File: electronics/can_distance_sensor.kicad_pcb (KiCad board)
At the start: 4 copper layers, 39.4 x 47.6 mm, 78 parts, among them J1 USB_B_Micro, J2 Conn_ARM_JTAG_SWD_10, J4 Conn_01x02_Socket, J5 Conn_01x04, Q1 IRLML6401, SW1 PTS645SK50SMTR92LFS, U1 USBLC6-2SC6, U2 STM32F446RETx, U3 LM1117DT-ADJ, U4 AOZ1280CI, U5 VL53L3CXV0DH/1, U6 TCAN1043xDxQ1, Y1 Crystal_GND24

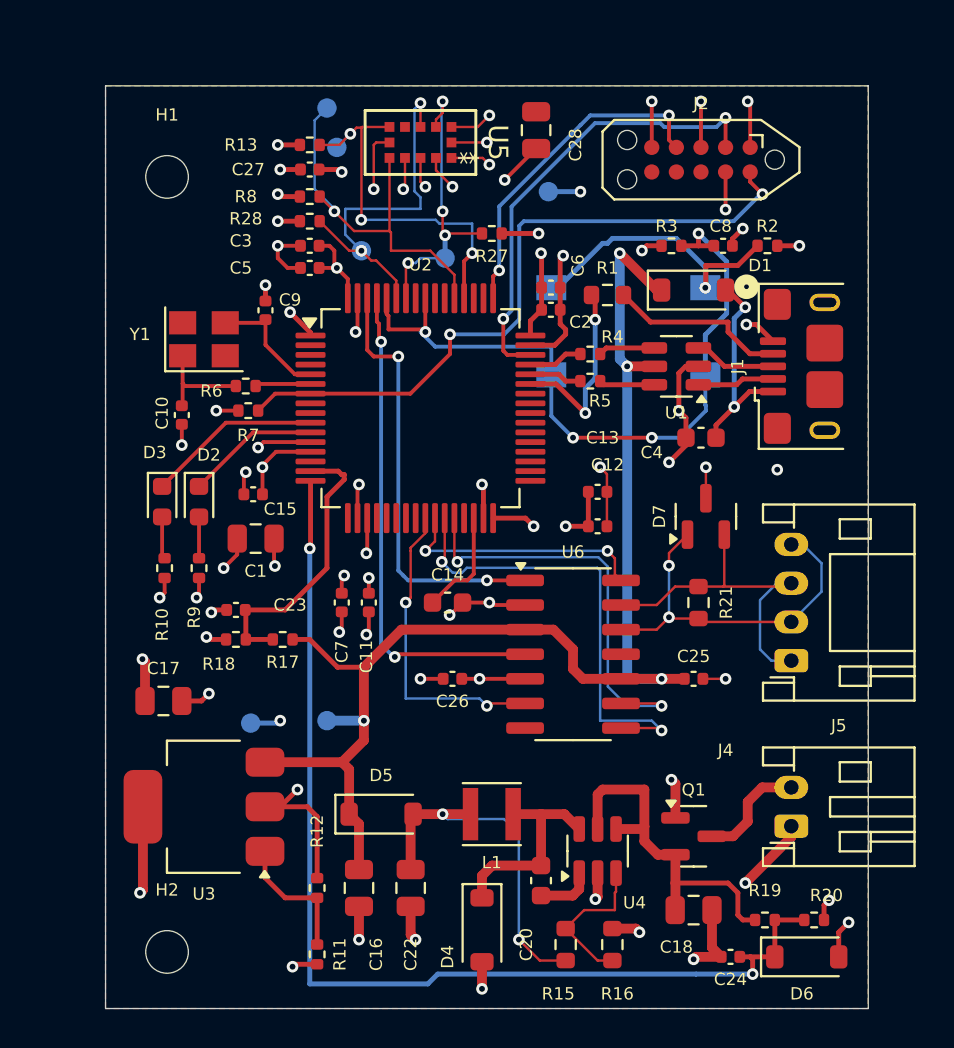
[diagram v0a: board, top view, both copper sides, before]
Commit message: Ordered this version.
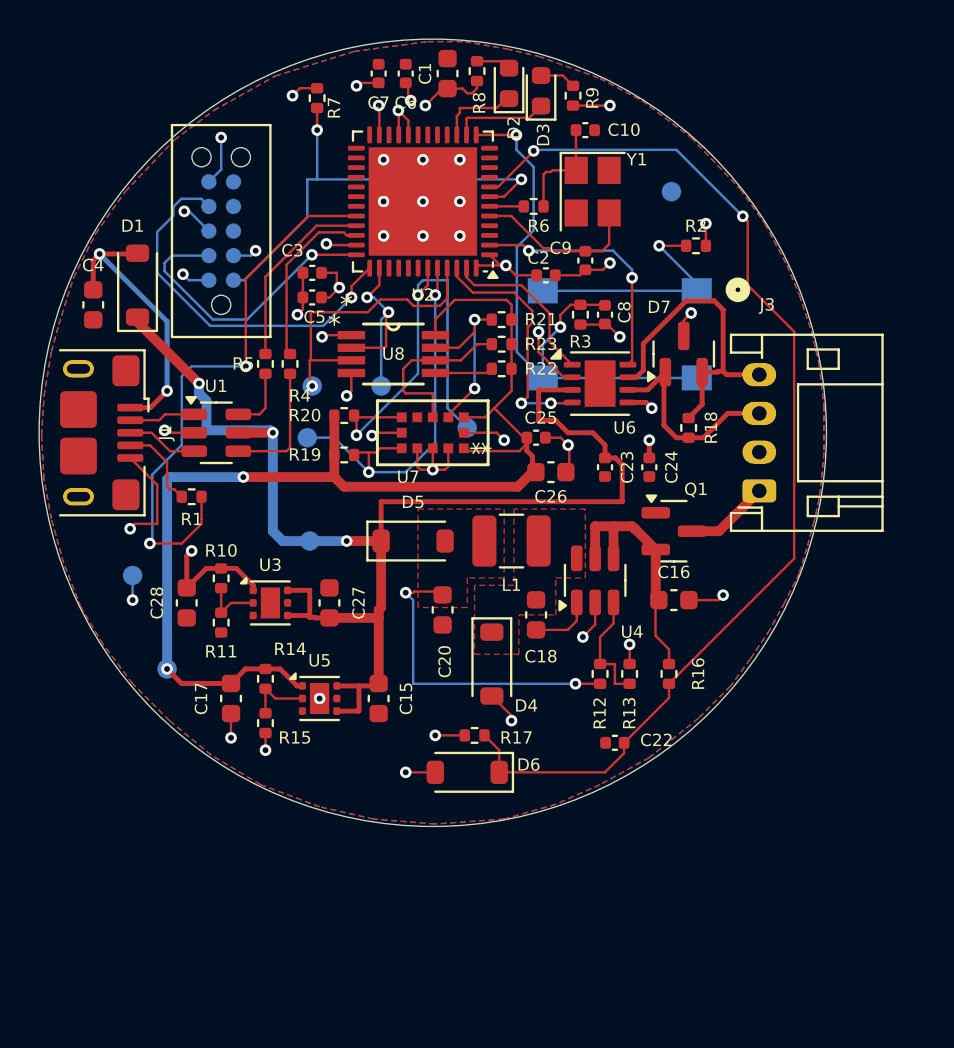
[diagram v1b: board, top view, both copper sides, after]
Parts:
- removed C11, C12, C13: 0.1u, Capacitor_SMD:C_0402_1005Metric
- removed C14: 2.2u, Capacitor_SMD:C_0603_1608Metric
- removed the C16 at (190.2, 129.2)
- removed the C23 at (183.9, 114.8)
- removed H1, H2: MountingHole, MountingHole:MountingHole_2.2mm_M2
- removed J4: Conn_01x02_Socket, Connector_JST:JST_PH_S2B-PH-K_1x02_P2.00mm_Horizontal
- removed the R12 at (188.1, 129.2)
- removed the R17 at (186.3, 116.3)
- removed the R18 at (183.9, 116.3)
- added C27: 4.7u, Capacitor_SMD:C_0603_1608Metric, F.Cu at (188.7, 114.4)
- added C28: 4.7u, Capacitor_SMD:C_0603_1608Metric, F.Cu at (181.4, 114.4)
- added R10: 5k, Resistor_SMD:R_0402_1005Metric, F.Cu at (183.1, 113.2)
- added R14: 4.09k, Resistor_SMD:R_0402_1005Metric, F.Cu at (185.4, 118.4)
- added R15: 1k, Resistor_SMD:R_0402_1005Metric, F.Cu at (185.4, 120.7)
- added R22: 10K, Resistor_SMD:R_0402_1005Metric, F.Cu at (197.6, 102.4)
- added TP8: TestPoint, TestPoint:TestPoint_Pad_D1.0mm, B.Cu at (180.3, 117.9)
- added U5: TLV75801PDRV, Package_SON:WSON-6-1EP_2x2mm_P0.65mm_EP1x1.6mm, F.Cu at (188.2, 119.4)
- added U8: TCA9509DGKR, footprints:DGK8, F.Cu at (192.0, 101.6)
- C1: footprint Capacitor_SMD:C_0805_2012Metric -> Capacitor_SMD:C_0603_1608Metric
- C15: value 0.1u -> 4.7u; footprint Capacitor_SMD:C_0402_1005Metric -> Capacitor_SMD:C_0603_1608Metric
- C16: renamed from C18; footprint Capacitor_SMD:C_0805_2012Metric -> Capacitor_SMD:C_0603_1608Metric
- C17: value 10u -> 4.7u; footprint Capacitor_SMD:C_0805_2012Metric -> Capacitor_SMD:C_0603_1608Metric
- C20: renamed from C22; footprint Capacitor_SMD:C_0805_2012Metric -> Capacitor_SMD:C_0603_1608Metric
- C26: renamed from C28; footprint Capacitor_SMD:C_0805_2012Metric -> Capacitor_SMD:C_0603_1608Metric
- J2: moved to B.Cu
- L1: footprint Inductor_SMD:L_Taiyo-Yuden_MD-3030 -> Inductor_SMD:L_1210_3225Metric
- R1: footprint Resistor_SMD:R_0603_1608Metric -> Resistor_SMD:R_0402_1005Metric
- R11: value 1.6k -> 1k
- R12: renamed from R15; footprint Resistor_SMD:R_0603_1608Metric -> Resistor_SMD:R_0402_1005Metric
- R13: renamed from R16; footprint Resistor_SMD:R_0603_1608Metric -> Resistor_SMD:R_0402_1005Metric
- R18: renamed from R21; footprint Resistor_SMD:R_0603_1608Metric -> Resistor_SMD:R_0402_1005Metric
- U2: value STM32F446RETx -> STM32G431CBUx; footprint Package_QFP:LQFP-64_10x10mm_P0.5mm -> Package_DFN_QFN:QFN-48-1EP_7x7mm_P0.5mm_EP5.6x5.6mm
- U3: value LM1117DT-ADJ -> TLV75801PDRV; footprint Package_TO_SOT_SMD:SOT-223-3_TabPin2 -> Package_SON:WSON-6-1EP_2x2mm_P0.65mm_EP1x1.6mm
- U6: value TCAN1043xDxQ1 -> TCAN1044A-Q1; footprint Package_SO:SOIC-14_3.9x8.7mm_P1.27mm -> Package_SON:VSON-8-1EP_3x3mm_P0.65mm_EP1.6x2.4mm
- moved J1 38.7 mm to (175.8, 105.7), turned to -90 degrees
- moved R9 32.2 mm to (201.3, 88.3)
- moved C4 32.1 mm to (176.5, 99.1), turned to 90 degrees
- moved R8 29.4 mm to (196.3, 87.0)
- moved D3 28.9 mm to (199.6, 88.0), turned to 90 degrees
- moved D1 28.7 mm to (178.8, 98.0), turned to 90 degrees
- moved C7 27.4 mm to (191.3, 87.1), turned to 90 degrees
- moved D2 26.9 mm to (198.0, 87.6), turned to 90 degrees
- moved C1 26.0 mm to (194.8, 87.1), turned to 90 degrees
- moved C10 25.5 mm to (201.9, 90.0), turned to 180 degrees
- moved J2 25.0 mm to (183.1, 95.2), turned to 90 degrees
- moved U1 24.0 mm to (182.9, 105.7), turned to 0 degrees
- moved R1 23.9 mm to (181.6, 109.0), turned to 180 degrees
- moved Y1 21.5 mm to (202.3, 93.2), turned to -90 degrees
- moved D6 19.9 mm to (195.8, 123.2), turned to 180 degrees
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- renumbered C20 to C18, C24 to C22, C25 to C23, C26 to C24, C27 to C25, J5 to J3, R19 to R16, R20 to R17, R8 to R19, R13 to R20, R27 to R21, R28 to R23, R9 to R8, R10 to R9, TP2 to TP1, TP4 to TP2, TP5 to TP3, TP6 to TP4, TP7 to TP5, TP1 to TP6, TP3 to TP7, U5 to U7
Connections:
- net Net-(D4-K) renamed /Power/LX
- net Net-(D5-A) renamed /Power/PRE_OUT
- C15 pad 1: 3V3 -> VCC
- C17 pad 1: 3V3 -> 2V8
- C25 pad 1: 3V3 -> 2V8
- C26 pad 1: 3V3 -> 2V8
- D7 pad 1: Net-(J5-Pin_2) -> Net-(J3-Pin_3)
- D7 pad 2: Net-(J5-Pin_1) -> Net-(J3-Pin_4)
- J3 pad 1: Net-(J5-Pin_1) -> VIN
- J3 pad 2: Net-(J5-Pin_2) -> GND
- J3 pad 3: Net-(J5-Pin_1) -> Net-(J3-Pin_3)
- J3 pad 4: Net-(J5-Pin_2) -> Net-(J3-Pin_4)
- Q1 pad 3: /Power/VIN -> VIN
- R11 pad 1: Net-(U3-ADJ) -> Net-(U3-FB)
- R18 pad 1: Net-(J5-Pin_1) -> Net-(J3-Pin_4)
- R18 pad 2: Net-(J5-Pin_2) -> Net-(J3-Pin_3)
- R19 pad 1: 3V3 -> 2V8
- R20 pad 1: 3V3 -> 2V8
- R21 pad 1: 3V3 -> 2V8
- R21 pad 2: TOF_SCL -> TOF_SCL_2V8
- R23 pad 1: 3V3 -> 2V8
- R23 pad 2: TOF_SDA -> TOF_SDA_2V8
- U2 pad 10: LED2 -> unconnected-(U2-PA2-Pad10)
- U2 pad 11: LED1 -> unconnected-(U2-PA3-Pad11)
- U2 pad 12: GND -> unconnected-(U2-PA4-Pad12)
- U2 pad 13: 3V3 -> BOOT
- U2 pad 14: ANALOG_IN -> LED2
- U2 pad 15: VCC_MEAS -> LED1
- U2 pad 16: VIN_MEAS -> unconnected-(U2-PC4-Pad16)
- U2 pad 18: GND -> unconnected-(U2-PB1-Pad18)
- U2 pad 19: 3V3 -> unconnected-(U2-PB2-Pad19)
- U2 pad 2: unconnected-(U2-PC13-Pad2) -> CAN_STB
- U2 pad 20: unconnected-(U2-PA4-Pad20) -> 3V3
- U2 pad 21: unconnected-(U2-PA5-Pad21) -> 3V3
- U2 pad 23: unconnected-(U2-PA7-Pad23) -> 3V3
- U2 pad 25: CAN_EN -> unconnected-(U2-PB12-Pad25)
- U2 pad 26: CAN_STB -> unconnected-(U2-PB13-Pad26)
- U2 pad 27: CAN_FAULT -> unconnected-(U2-PB14-Pad27)
- U2 pad 28: CAN_WAKE -> unconnected-(U2-PB15-Pad28)
- U2 pad 30: Net-(U2-VCAP_1) -> unconnected-(U2-PA8-Pad30)
- U2 pad 31: GND -> unconnected-(U2-PA9-Pad31)
- U2 pad 32: 3V3 -> ID
- U2 pad 33: unconnected-(U2-PB12-Pad33) -> DM
- U2 pad 34: unconnected-(U2-PB13-Pad34) -> DP
- U2 pad 35: unconnected-(U2-PB14-Pad35) -> 3V3
- U2 pad 36: unconnected-(U2-PB15-Pad36) -> SWDIO
- U2 pad 37: unconnected-(U2-PC6-Pad37) -> SWCLK
- U2 pad 38: unconnected-(U2-PC7-Pad38) -> TOF_SCL
- U2 pad 43: ID -> TOF_INT
- U2 pad 44: DM -> TOF_XSHUT
- U2 pad 45: DP -> TOF_SDA
- U2 pad 46: SWDIO -> CAN_RX
- U2 pad 47: GND -> CAN_TX
- U2 pad 49: SWCLK -> GND
- U2 pad 8: unconnected-(U2-PC0-Pad8) -> VIN_MEAS
- U3 pad 1: Net-(U3-ADJ) -> 3V3
- U3 pad 2: 3V3 -> Net-(U3-FB)
- U3 pad 3: VCC -> GND
- U6 pad 6: CAN_EN -> Net-(J3-Pin_3)
- U6 pad 7: unconnected-(U6-INH-Pad7) -> Net-(J3-Pin_4)
- U6 pad 8: CAN_FAULT -> CAN_STB
- U6 pad 9: CAN_WAKE -> (no net)
- U7 pad 1: 3V3 -> 2V8
- U7 pad 10: TOF_SCL -> TOF_SCL_2V8
- U7 pad 11: 3V3 -> 2V8
- U7 pad 9: TOF_SDA -> TOF_SDA_2V8
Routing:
- net 2V8: track 0.00 -> 61.0 mm, vias 0 -> 2
- net GND: track 91.6 -> 49.1 mm, vias 48 -> 33
- net 3V3: track 65.1 -> 36.2 mm, vias 28 -> 17
- net CAN_FAULT: track 24.2 -> 0.00 mm, vias 2 -> 0
- net CAN_WAKE: track 21.9 -> 0.00 mm, vias 2 -> 0
- net Net-(J5-Pin_2): track 19.5 -> 0.00 mm, vias 2 -> 0
- net ID: track 9.84 -> 28.9 mm
- net Net-(J5-Pin_1): track 18.3 -> 0.00 mm
- net Net-(J3-Pin_4): track 0.00 -> 16.4 mm
- net CAN_EN: track 16.1 -> 0.00 mm, vias 2 -> 0
- net VCC_MEAS: track 15.0 -> 0.00 mm
- net CAN_TX: track 22.2 -> 8.67 mm, vias 2 -> 0
- net CAN_RX: track 25.7 -> 12.7 mm
- net NRST: track 35.5 -> 23.9 mm
- net /Power/LX: track 10.8 -> 0.00 mm
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- added copper zone on F.Cu, net /Power/LX
- added copper zone on F.Cu, net /Power/PRE_OUT
- added copper zone on B.Cu, net GND
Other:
- board size 39.4 x 47.6 mm -> 40.6 x 40.6 mm
- board text added: "TP1 = 3.3V TP2 = TOF_SDA TP3 = VCC TP4 = TOF_SCL TP5 = TOF_INT TP6 = TOF_XSHUT TP7 = GND"
- board text removed: "TP1 = 3.3V TP2 = TOF_SDA TP3 = VCC TP4 = TOF_SCL TP5 = TOF_INT TP6 = TOF_RST TP7 = GND"
